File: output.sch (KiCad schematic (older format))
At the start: 6 parts, among them P14 SERVO_OUT_0, P15 SERVO_OUT_1, P16 SERVO_OUT_2, P17 SERVO_OUT_3, P18 SERVO_OUT_4, P19 SERVO_OUT_5

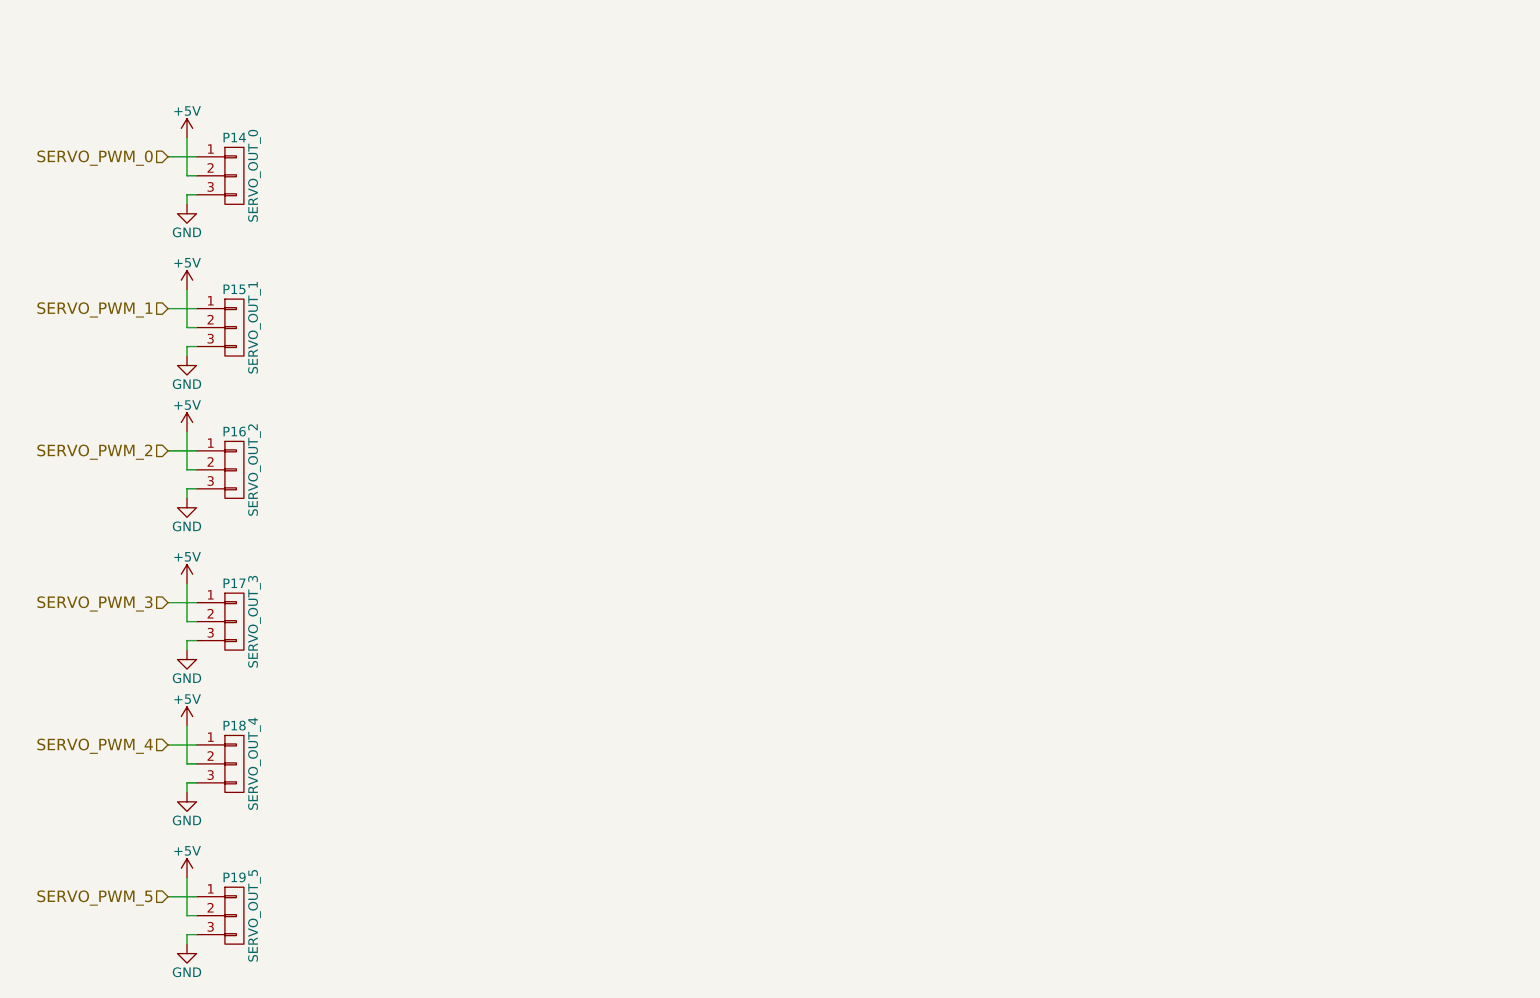
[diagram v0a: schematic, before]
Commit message: PCB rev1.0
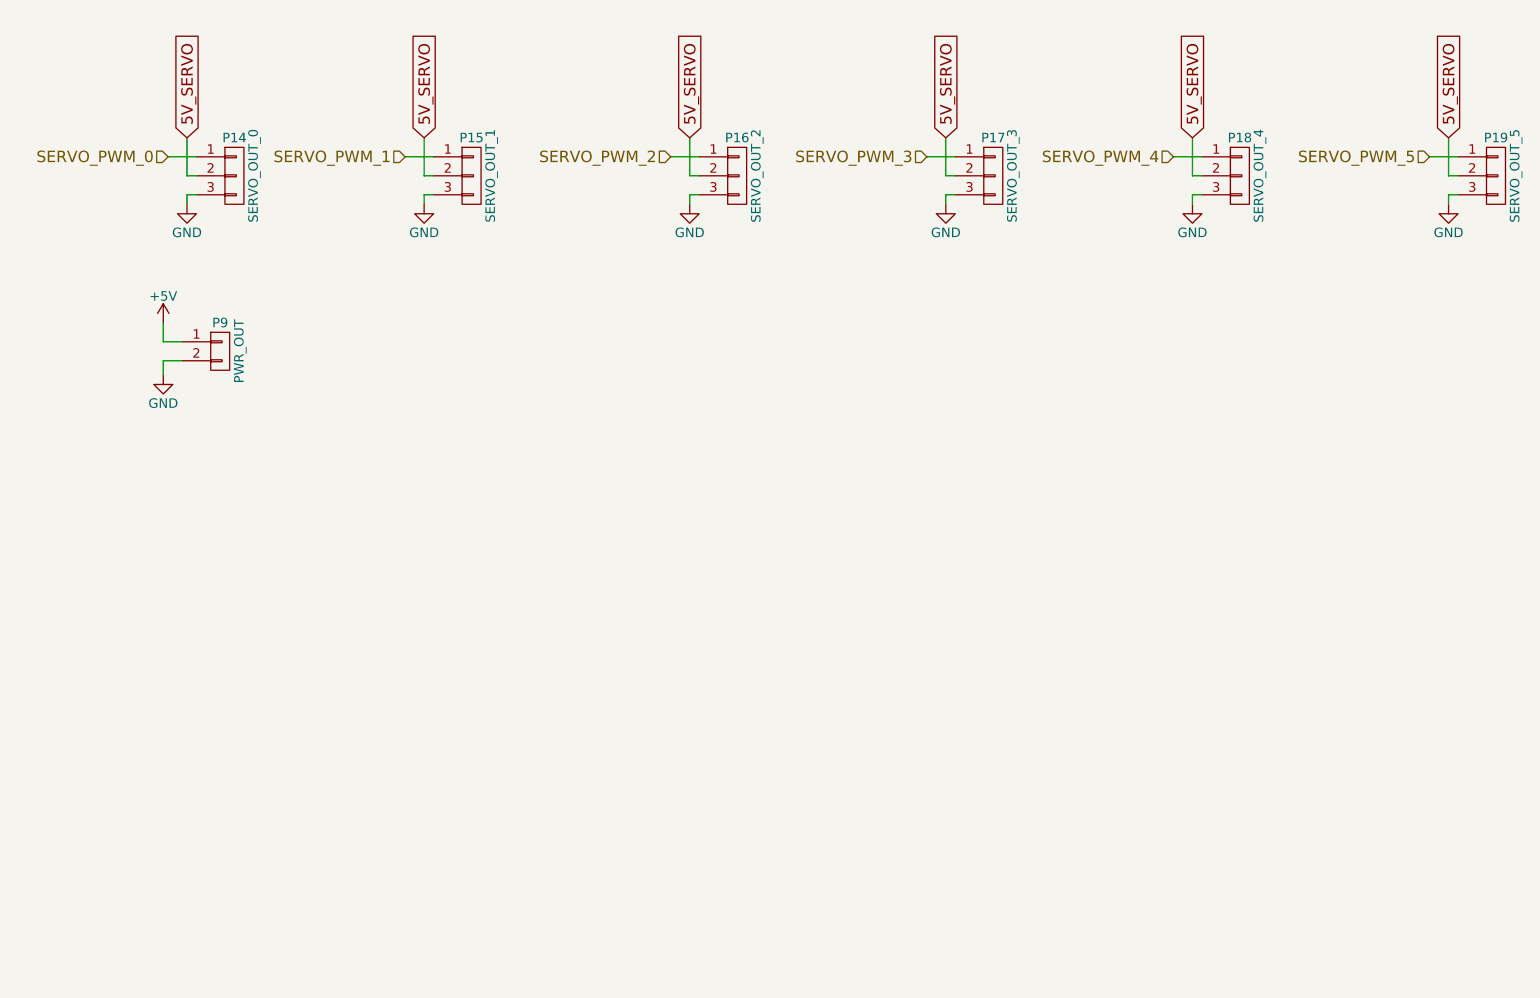
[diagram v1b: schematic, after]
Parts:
- added P9: PWR_OUT, Socket_Strips:Socket_Strip_Straight_1x02, symbol CONN_01X02
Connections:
- net +5V: now also P9.1 (P1); no longer P14.2 (P2), P15.2 (P2), P16.2 (P2), P17.2 (P2), P18.2 (P2), P19.2 (P2)
- net GND: now also P9.2 (P2)
- new net 5V_SERVO: P14.2 (P2), P15.2 (P2), P16.2 (P2), P17.2 (P2), P18.2 (P2), P19.2 (P2)
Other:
- moved on the sheet: P15, P16, P17, P18, P19
